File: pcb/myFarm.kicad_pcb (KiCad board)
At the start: 2 copper layers, 63.5 x 52.1 mm, 10 parts, among them J0 Conn_01x02, J1 LED, J2 SENSOR, J3 SW_LED, J4 RELAY, J5 POWER DRIVE, J6 JUMPER, J7 SW_LED, U1 WeMos_D1_mini, U2 MCP23017_MODULE

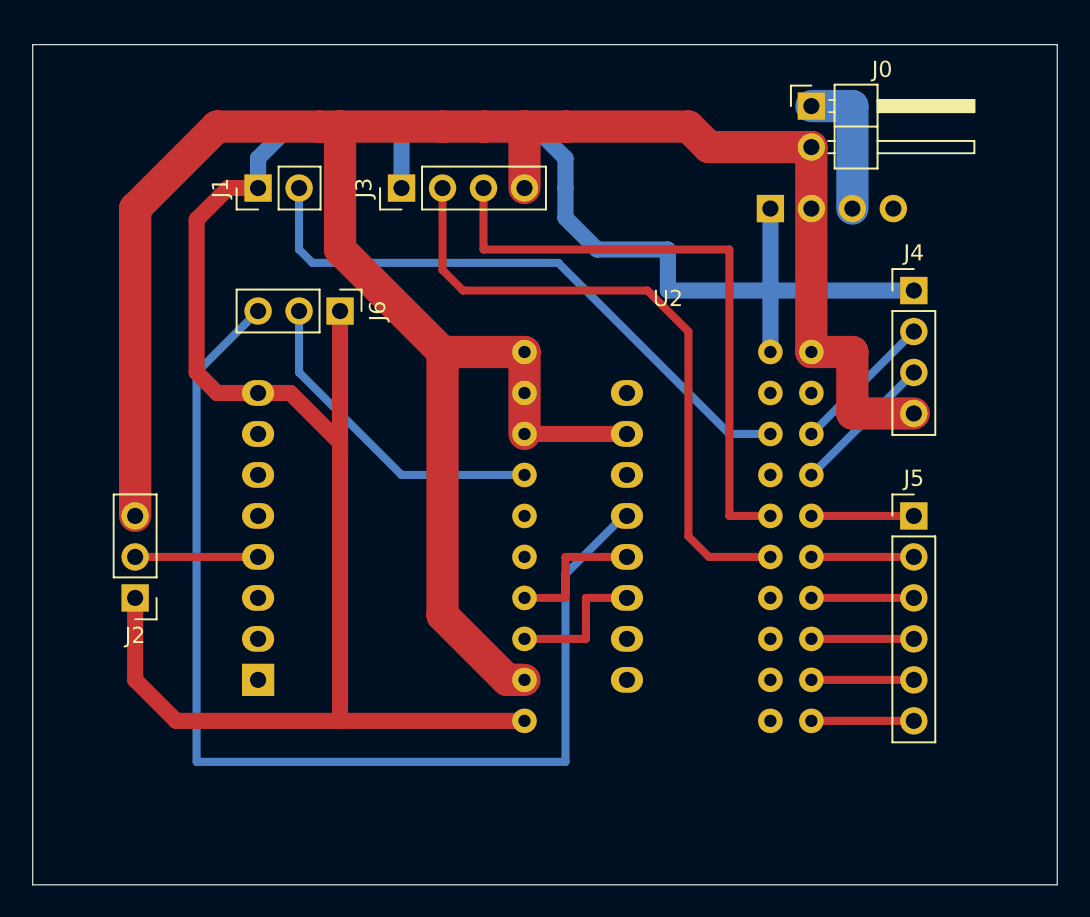
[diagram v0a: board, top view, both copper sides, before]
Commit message: update pcb
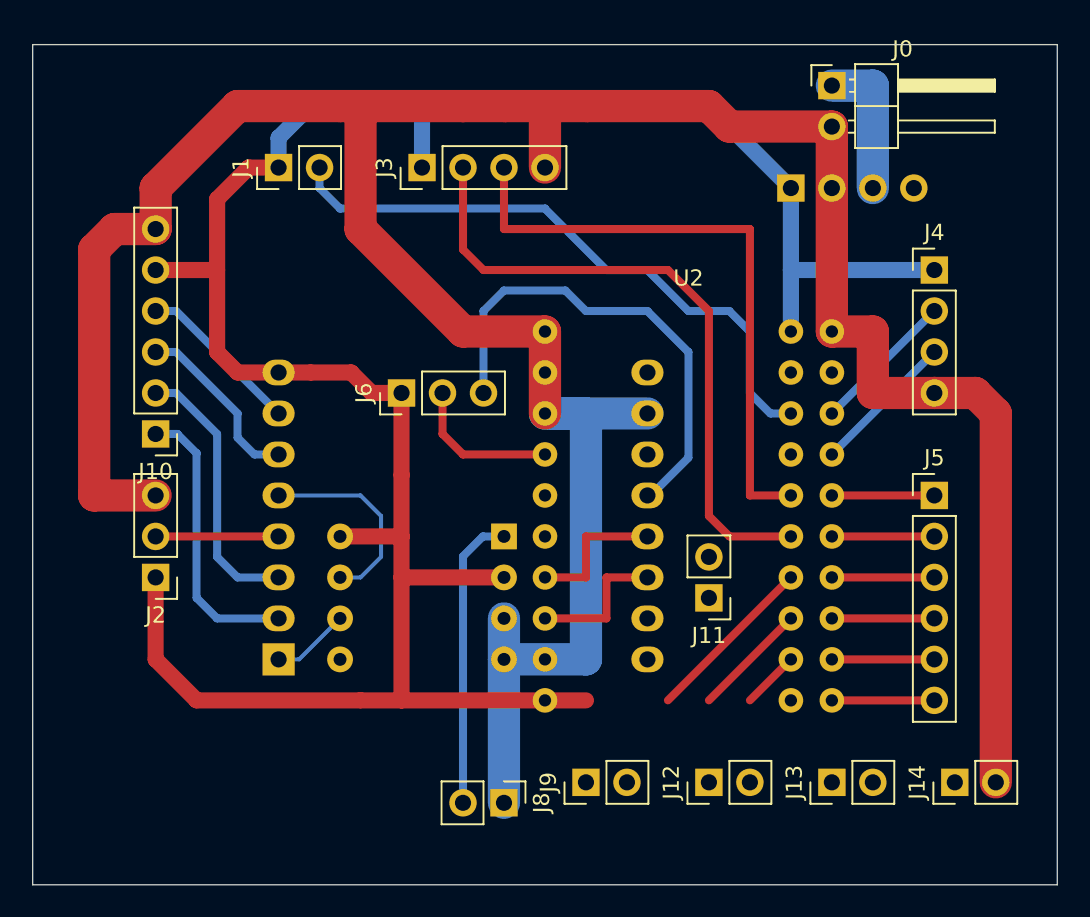
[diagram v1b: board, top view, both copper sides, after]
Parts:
- added J10: GENERAL, Connector_PinHeader_2.54mm:PinHeader_1x06_P2.54mm_Vertical, F.Cu at (69.8, 72.4)
- added J11: RXTX, Connector_PinHeader_2.54mm:PinHeader_1x02_P2.54mm_Vertical, F.Cu at (104.1, 82.5)
- added J12: VALVE OUT, Connector_PinHeader_2.54mm:PinHeader_1x02_P2.54mm_Vertical, F.Cu at (104.1, 94.0)
- added J13: VALVE OUT, Connector_PinHeader_2.54mm:PinHeader_1x02_P2.54mm_Vertical, F.Cu at (111.8, 94.0)
- added J14: VALVE OUT, Connector_PinHeader_2.54mm:PinHeader_1x02_P2.54mm_Vertical, F.Cu at (119.4, 94.0)
- added J8: Reset, Connector_PinHeader_2.54mm:PinHeader_1x02_P2.54mm_Vertical, F.Cu at (91.4, 95.2)
- added J9: VAVLE IN, Connector_PinHeader_2.54mm:PinHeader_1x02_P2.54mm_Vertical, F.Cu at (96.5, 94.0)
- added U3: DS1832S+, Package_DIP:DIP-8_W10.16mm, B.Cu at (91.4, 78.7)
- J0: value Conn_01x02 -> POWER
- J7: value SW_LED -> SUPPLY
- moved J6 6.35 mm to (85.1, 69.8), turned to 90 degrees
- moved J0 1.80 mm to (111.8, 50.8)
- moved U2 1.80 mm to (102.9, 62.2)
- moved J4 1.80 mm to (118.1, 62.2)
- moved J7 1.80 mm to (109.2, 57.1)
- moved J1 1.80 mm to (77.5, 55.9)
- moved J2 1.80 mm to (69.8, 81.3)
- moved J3 1.80 mm to (86.4, 55.9)
- moved J5 1.80 mm to (118.1, 76.2)
- moved U1 1.80 mm to (77.5, 86.4)
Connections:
- U1 pad 1: (no net) -> Net-(U1-Pad1)
- U1 pad 15: (no net) -> Net-(J11-Pad2)
- U1 pad 16: (no net) -> Net-(J11-Pad1)
- U1 pad 2: (no net) -> Net-(J10-Pad1)
- U1 pad 3: (no net) -> Net-(J10-Pad2)
- U1 pad 5: (no net) -> Net-(U1-Pad5)
- U1 pad 6: (no net) -> Net-(J10-Pad3)
- U1 pad 7: (no net) -> Net-(J10-Pad4)
- U2 pad 5: (no net) -> Net-(J9-Pad1)
- U2 pad 6: (no net) -> Net-(J12-Pad1)
- U2 pad 7: (no net) -> Net-(J13-Pad1)
- U2 pad 8: (no net) -> Net-(J14-Pad1)
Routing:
- net GNDREF: track 146.4 -> 191.7 mm
- net Net-(J6-Pad3): track 69.3 -> 30.1 mm
- net Net-(J8-Pad2): track 0.00 -> 18.3 mm
- net Net-(J10-Pad1): track 0.00 -> 17.6 mm
- net Net-(J10-Pad2): track 0.00 -> 16.8 mm
- net Net-(U1-Pad5): track 0.00 -> 12.5 mm
- net Net-(J10-Pad3): track 0.00 -> 11.1 mm
- net Net-(J6-Pad2): track 20.4 -> 9.42 mm
- net Net-(J9-Pad1): track 0.00 -> 10.8 mm
- net Net-(J10-Pad4): track 0.00 -> 10.3 mm
- net Net-(J12-Pad1): track 0.00 -> 7.18 mm
- net Net-(J1-Pad1): track 145.0 -> 150.5 mm
- net Net-(U1-Pad1): track 0.00 -> 4.86 mm
- net Net-(J13-Pad1): track 0.00 -> 3.59 mm
- net Net-(J1-Pad2): track 37.8 -> 38.5 mm
